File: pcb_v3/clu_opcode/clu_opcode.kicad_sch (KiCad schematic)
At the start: 44 parts, among them J2 Conn_01x09, J3 Conn_01x09

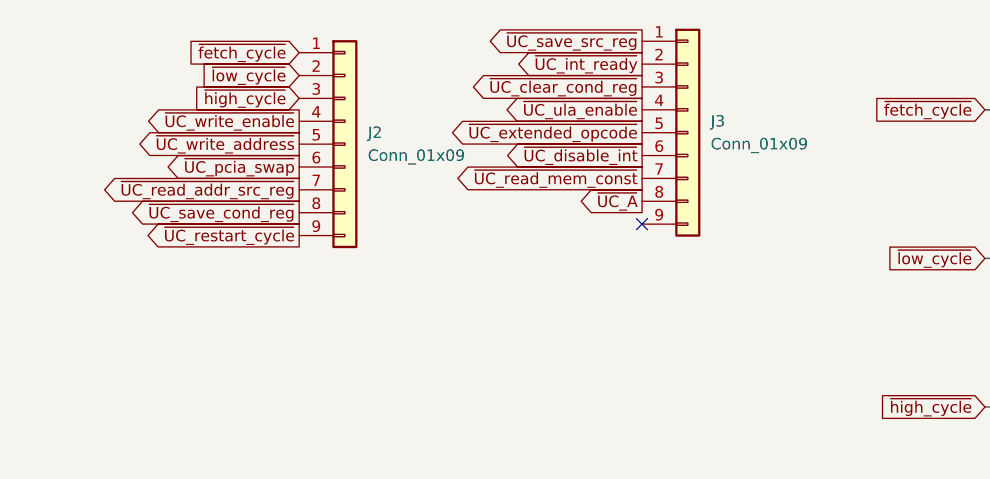
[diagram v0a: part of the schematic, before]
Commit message: .
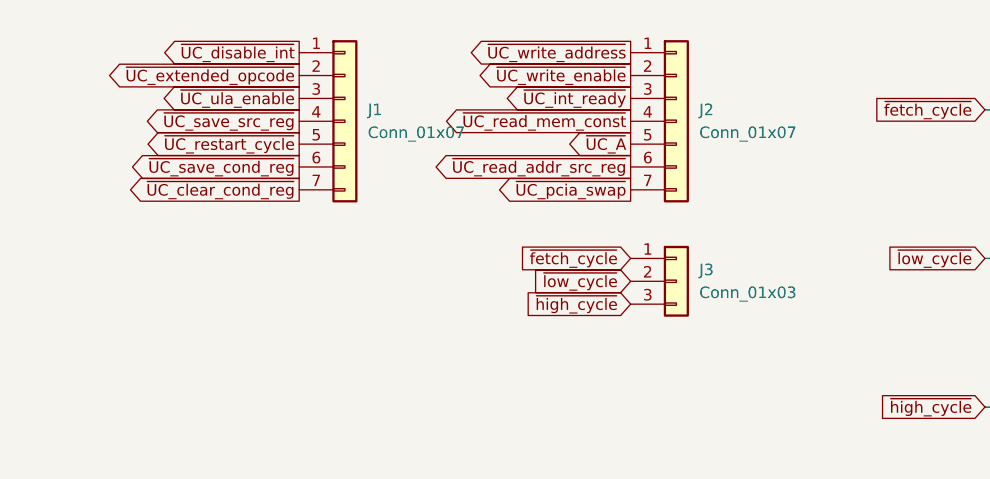
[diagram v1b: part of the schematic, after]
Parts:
- removed J2, J3: Conn_01x09, Connector_PinHeader_2.54mm:PinHeader_1x09_P2.54mm_Vertical, symbol Connector_Generic:Conn_01x09
- added J1, J2: Conn_01x07, Connector_PinHeader_2.54mm:PinHeader_1x07_P2.54mm_Vertical, symbol Connector_Generic:Conn_01x07
- added J3: Conn_01x03, Connector_PinHeader_2.54mm:PinHeader_1x03_P2.54mm_Vertical, symbol Connector_Generic:Conn_01x03
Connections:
- net ~{UC_A}: now also J2.5 (Pin_5)
- net ~{UC_clear_cond_reg}: now also J1.7 (Pin_7)
- net ~{UC_disable_int}: now also J1.1 (Pin_1)
- net ~{UC_extended_opcode}: now also J1.2 (Pin_2)
- net ~{UC_int_ready}: now also J2.3 (Pin_3)
- net ~{UC_pcia_swap}: now also J2.7 (Pin_7)
- net ~{UC_read_addr_src_reg}: now also J2.6 (Pin_6)
- net ~{UC_read_mem_const}: now also J2.4 (Pin_4)
- net ~{UC_restart_cycle}: now also J1.5 (Pin_5)
- net ~{UC_save_cond_reg}: now also J1.6 (Pin_6)
- net ~{UC_save_src_reg}: now also J1.4 (Pin_4)
- net ~{UC_ula_enable}: now also J1.3 (Pin_3)
- net ~{UC_write_address}: now also J2.1 (Pin_1)
- net ~{UC_write_enable}: now also J2.2 (Pin_2)
- net ~{fetch_cycle}: now also J3.1 (Pin_1)
- net ~{high_cycle}: now also J3.3 (Pin_3)
- net ~{low_cycle}: now also J3.2 (Pin_2)
- no-connect marks 1 -> 0
